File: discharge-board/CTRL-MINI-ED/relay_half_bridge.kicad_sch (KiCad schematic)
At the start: 10 parts, among them K1 G2RL-1A-E, K2 G2RL-1A-E, Q1 Q_NMOS_GSD, Q2 Q_NMOS_GSD

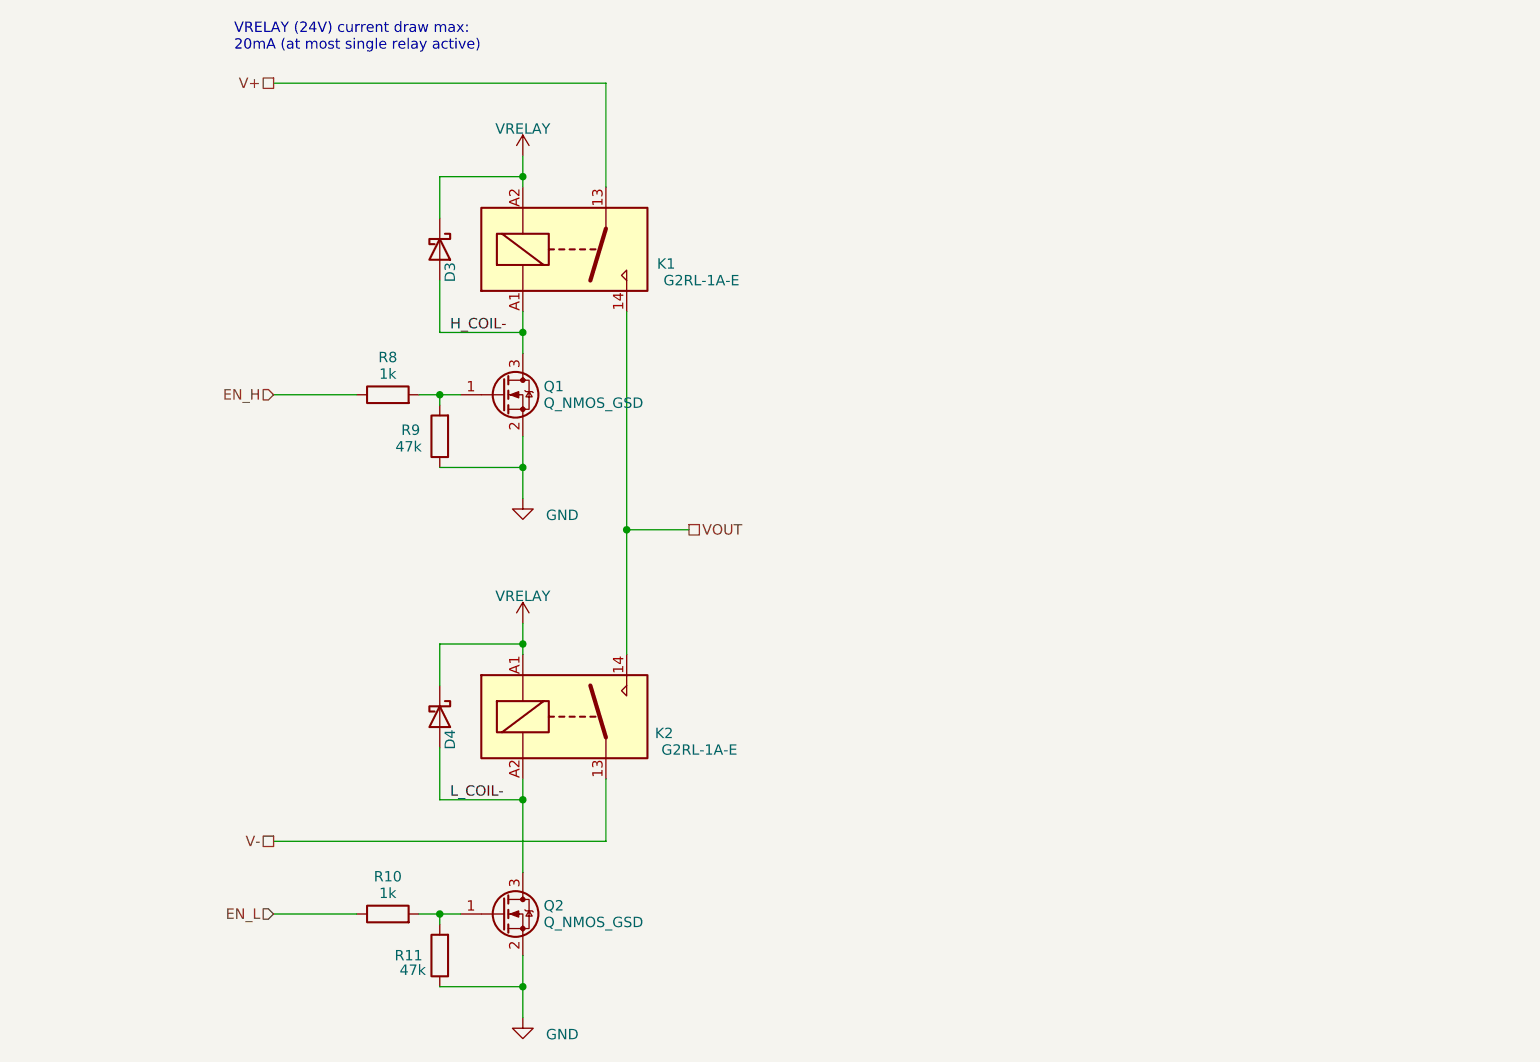
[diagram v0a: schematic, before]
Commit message: Draft of PCB layout
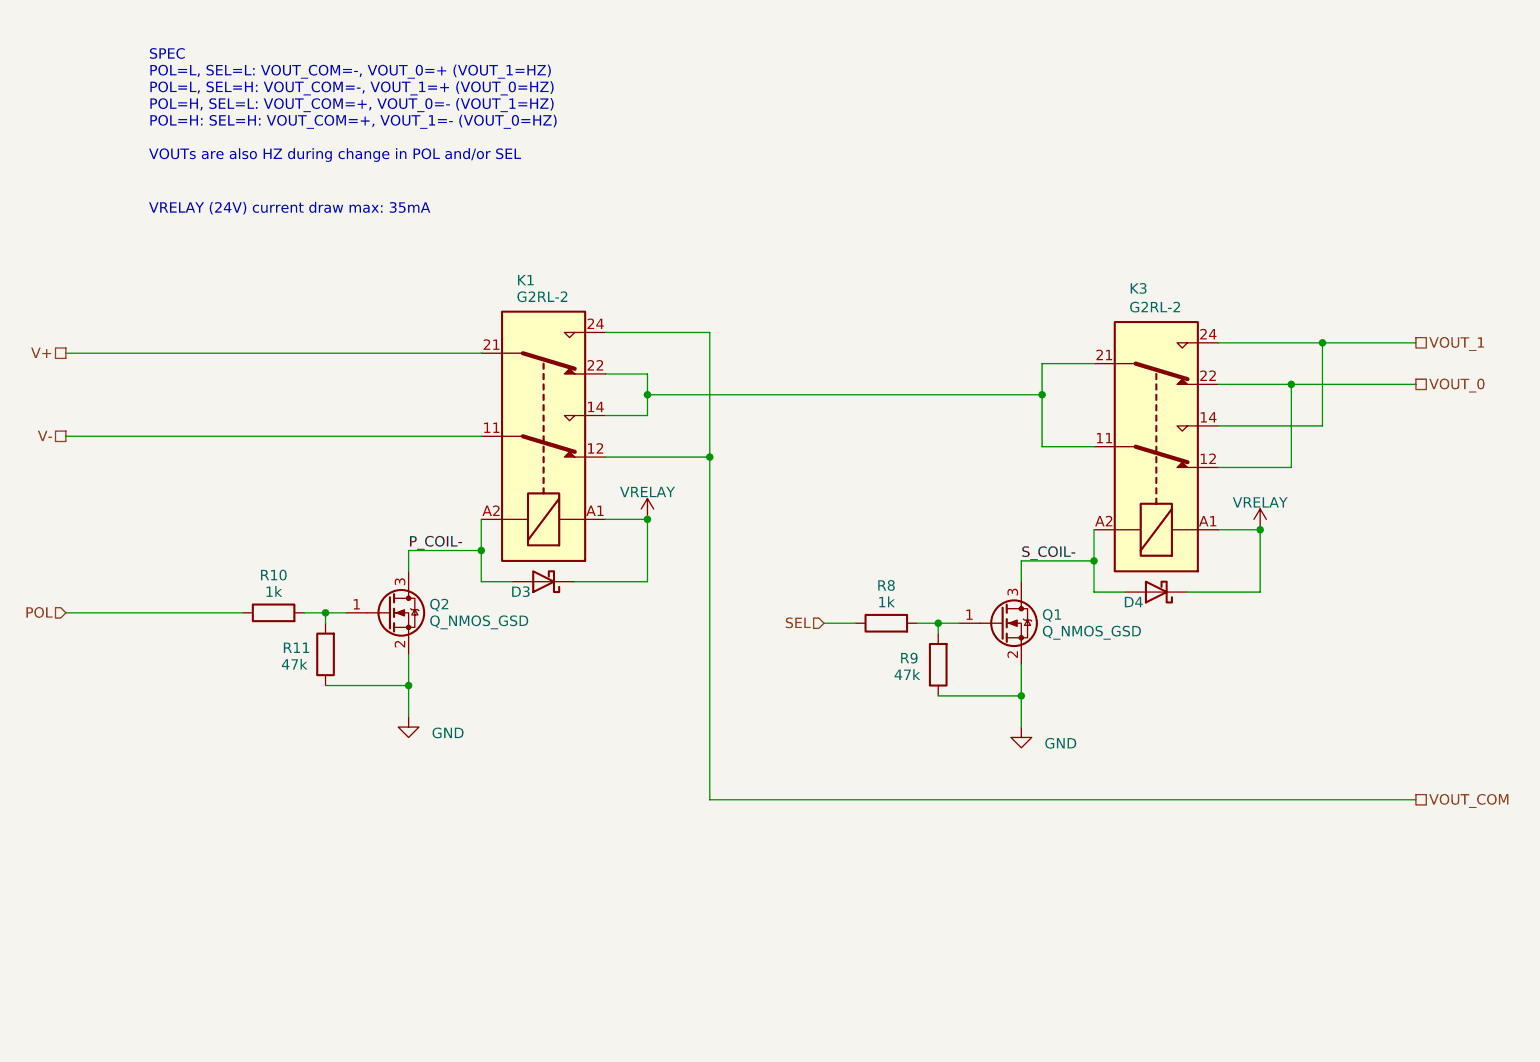
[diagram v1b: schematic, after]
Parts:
- removed K1, K2: G2RL-1A-E, Relay_THT:Relay_SPST_Omron_G2RL-1A-E, symbol Relay:G2RL-1A-E
- added K1, K3: G2RL-2, Relay_THT:Relay_DPDT_Omron_G2RL-2, symbol Relay:G2RL-2
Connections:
- net V+: now also K1.21
- net V-: now also K1.11
- net VRELAY: now also K1.A1, K3.A1
- net EN_H renamed SEL
- net EN_L renamed POL
- net H_COIL- renamed P_COIL-
- net P_COIL-: now also Q2.3 (D), K1.A2; no longer Q1.3 (D)
- net L_COIL- renamed S_COIL-
- net S_COIL-: now also Q1.3 (D), K3.A2; no longer Q2.3 (D)
- new net: K1.14, K1.22, K3.11, K3.21
- new net VOUT_0: K3.12, K3.22
- new net VOUT_1: K3.14, K3.24
- new net VOUT_COM: K1.12, K1.24
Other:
- note added: "SPEC POL=L, SEL=L: VOUT_COM=-, VOUT_0=+ (VOUT_1=HZ) POL=L, SEL=H: VOUT_COM=-, VOUT_1=+ (VOUT_0=HZ) POL=H, SEL=L: VOUT_COM=+, VOUT_0=- (VOUT_1=HZ) POL=H: SEL=H: VOUT_COM=+, VOUT_1=- (VOUT_0=HZ) VOUTs are also HZ during change in POL and/or SEL"
- note added: "VRELAY (24V) current draw max: 35mA"
- note removed: "VRELAY (24V) current draw max: 20mA (at most single relay active)"
